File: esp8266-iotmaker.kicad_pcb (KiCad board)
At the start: 2 copper layers, 66.3 x 30.7 mm, 70 parts, among them J1 CONN_01X04, J2 CONN_01X02, J3 CONN_01X08, J4 CONN_01X06, J5 CONN_01X08, J6 CONN_01X04, Q1 S8050, Q2 S8050, SW1 SW_Push, SW2 SW_Push, U1 usb_mini_b, U2 chip-esp8266, U3 CP2102, U4 25Q32, U5 mcp73831, U6 AMS1117-3.3, U7 AMS1117-3.3, U8 MOSFET-P, Y1 26MHz

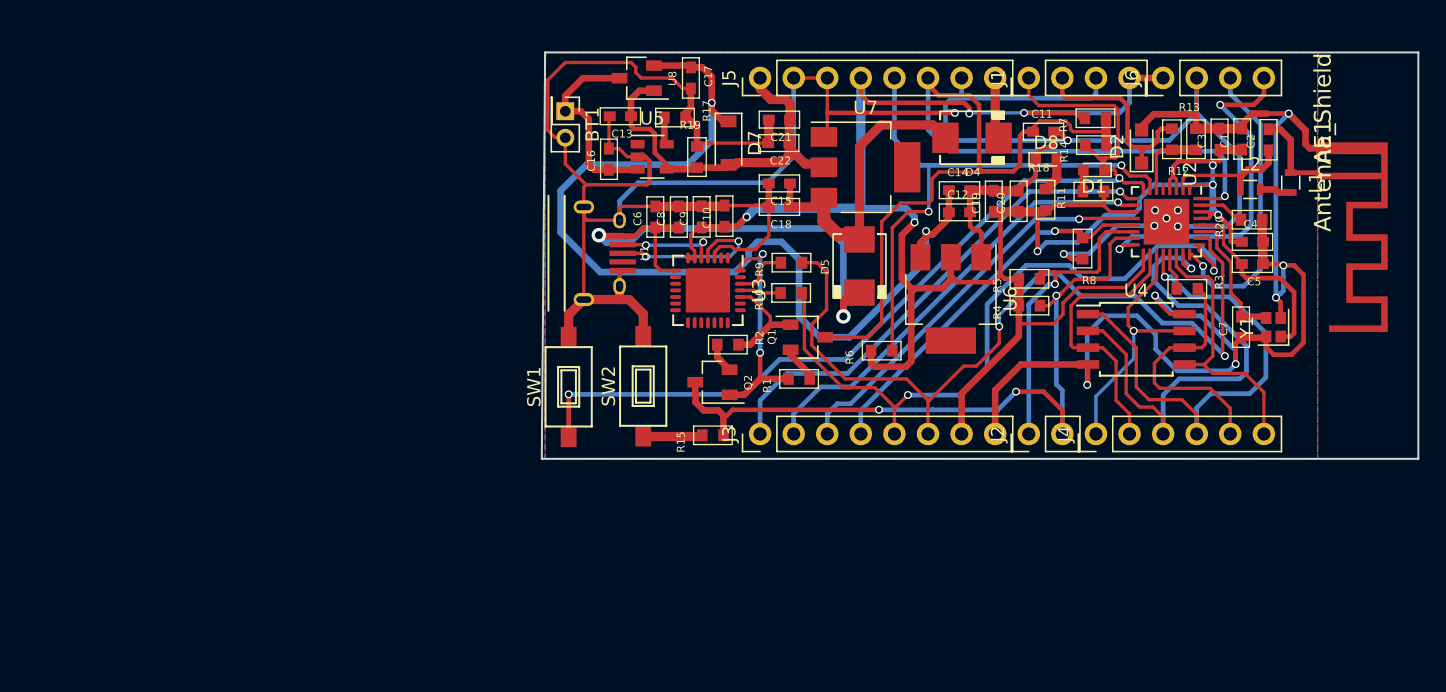
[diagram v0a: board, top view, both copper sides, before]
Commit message: complete pcb source
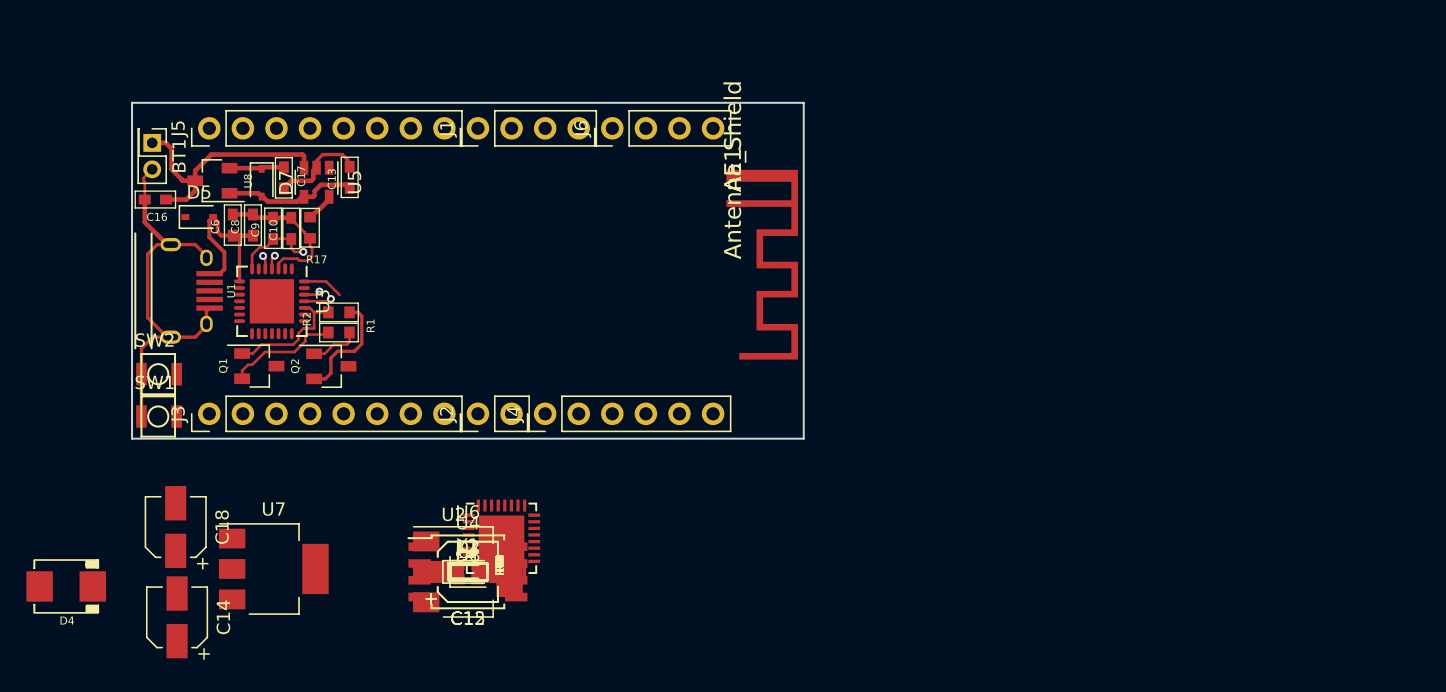
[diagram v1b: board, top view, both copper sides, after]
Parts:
- removed C19, C20, C21, C22: C, esp8266:C_0603
- C12, C14: value C -> 10uF; footprint esp8266:C_0603 -> Capacitors_SMD:CP_Elec_4x5.3
- C15, C18: value C -> 22uF; footprint esp8266:C_0603 -> Capacitors_SMD:CP_Elec_4x5.3
- D5: footprint esp8266:do214aa-g -> Diodes_SMD:D_SOD-323
- D7: footprint Diodes_SMD:D_SOD-123 -> Diodes_SMD:D_SOD-323
- SW1, SW2: footprint esp8266:Tact_Switch_TS6X3.6 -> esp8266:micro-buttom
- moved D4 76.5 mm to (90.8, 124.1)
- moved L1 68.8 mm to (121.2, 123.0), turned to 0 degrees
- moved C2 68.8 mm to (121.2, 123.0), turned to 0 degrees
- moved C14 67.4 mm to (99.2, 126.4), turned to 90 degrees
- moved C1 67.1 mm to (121.2, 123.0), turned to 0 degrees
- moved L2 65.9 mm to (121.2, 123.0)
- moved C3 65.6 mm to (121.2, 123.0), turned to 0 degrees
- moved R20 65.0 mm to (121.2, 123.0), turned to 0 degrees
- moved C4 64.4 mm to (121.2, 123.0)
- moved R13 64.1 mm to (121.2, 123.0), turned to 0 degrees
- moved C5 63.7 mm to (121.2, 123.0), turned to 0 degrees
- moved Y1 63.7 mm to (121.2, 123.0), turned to 0 degrees
- moved R12 62.5 mm to (121.2, 123.0), turned to 0 degrees
- moved C7 61.3 mm to (121.2, 123.0), turned to 0 degrees
- moved D2 60.3 mm to (121.2, 123.0), turned to 0 degrees
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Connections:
- C14 pad 1: VBAT -> Net-(C14-Pad1)
- C15 pad 1: Net-(C15-Pad1) -> 3V3
- C18 pad 1: Net-(C15-Pad1) -> 5V
- D4 pad 1: Net-(C15-Pad1) -> Net-(C14-Pad1)
- D5 pad 1: Net-(C15-Pad1) -> Net-(C14-Pad1)
- U7 pad 3: Net-(C15-Pad1) -> Net-(C14-Pad1)
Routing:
- net GND: track 325.7 -> 50.3 mm, vias 14 -> 0
- net 3V3: track 174.2 -> 6.35 mm, vias 8 -> 1
- net REST: track 80.4 -> 0.00 mm, vias 1 -> 0
- net GPIO16: track 72.7 -> 0.00 mm, vias 2 -> 0
- net VBAT: track 74.8 -> 4.18 mm, vias 2 -> 0
- net TXD: track 61.7 -> 0.00 mm, vias 2 -> 0
- net GPIO0: track 56.2 -> 0.00 mm, vias 3 -> 0
- net RXD: track 51.7 -> 0.00 mm, vias 2 -> 0
- net EN: track 42.1 -> 0.00 mm, vias 2 -> 0
- net MOSI: track 38.4 -> 0.00 mm, vias 1 -> 0
- net GPIO14: track 37.6 -> 0.00 mm, vias 1 -> 0
- net CSO: track 37.2 -> 0.00 mm, vias 1 -> 0
- net GPIO12: track 34.0 -> 0.00 mm, vias 1 -> 0
- net GPIO13: track 30.8 -> 0.00 mm, vias 1 -> 0
- net GPIO15: track 28.9 -> 0.00 mm, vias 1 -> 0
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- removed copper zone on B.Cu, net GND
- removed copper zone on F.Cu, net GND
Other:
- board size 66.3 x 30.7 mm -> 50.8 x 25.4 mm
- net class Default: trace_width 0.254 -> 0.2; via_dia 1.1 -> 1; via_drill 0.6 -> 0.5
